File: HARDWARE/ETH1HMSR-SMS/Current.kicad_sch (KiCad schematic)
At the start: 28 parts, among them J501 1710072, U501 HMSR-SMS, U502 DG419LDY, U503 DG411LEDQ, U504 OPA341UA, U505 OPA341UA

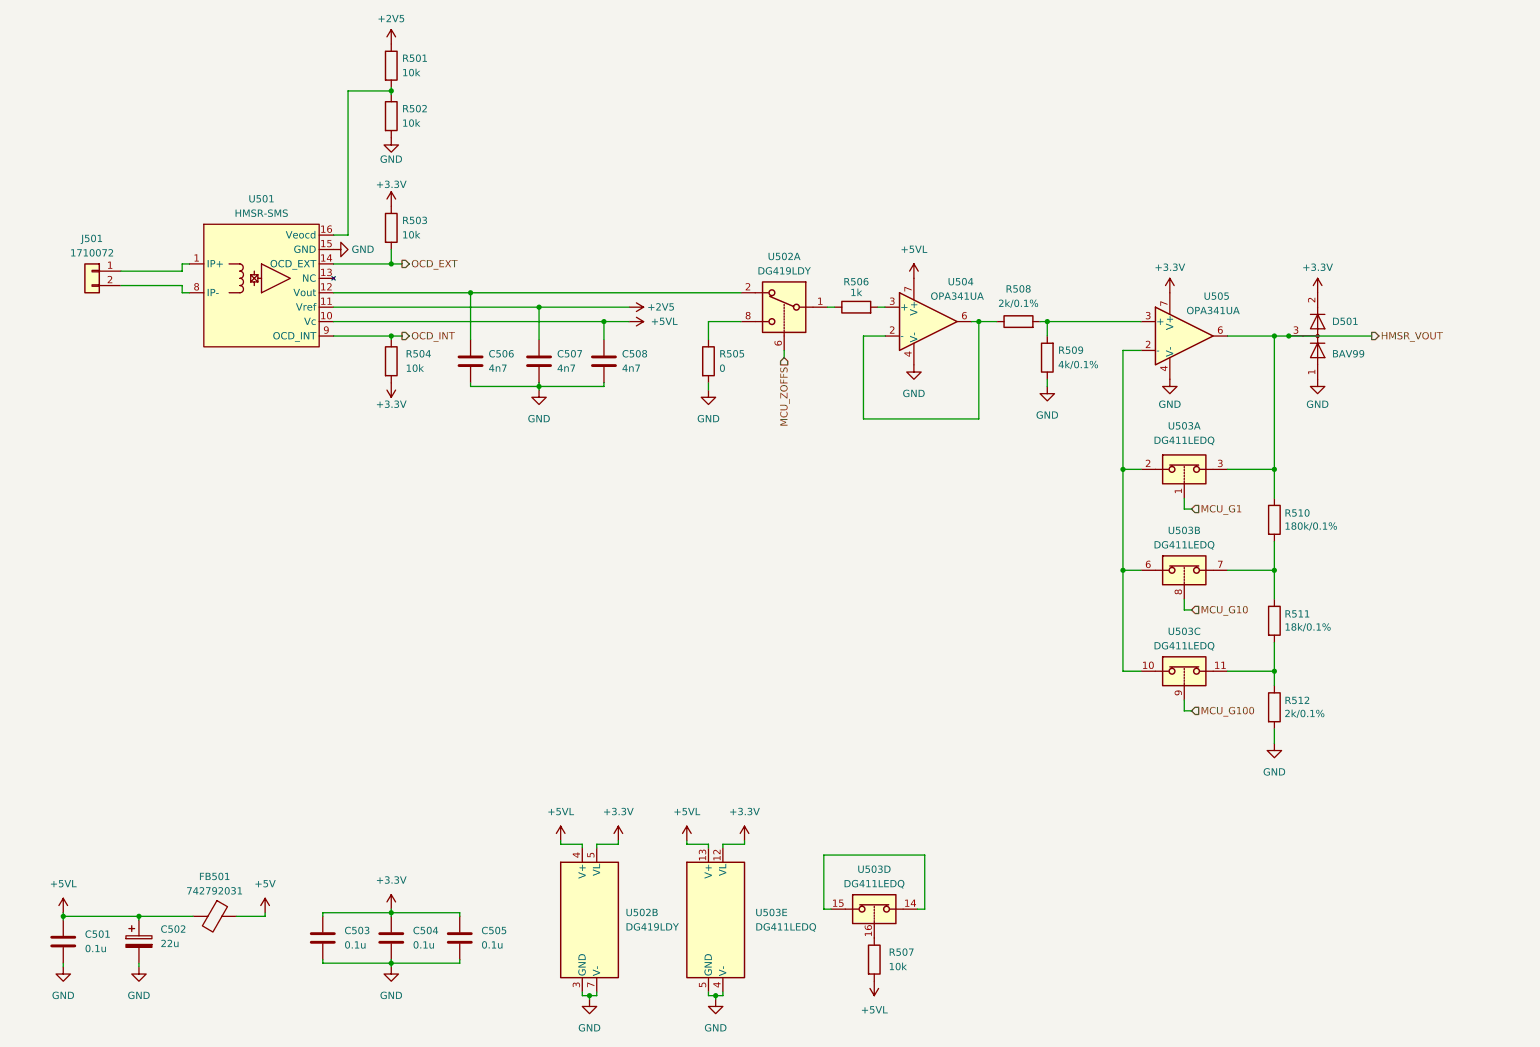
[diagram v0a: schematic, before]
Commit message: SW and HW development
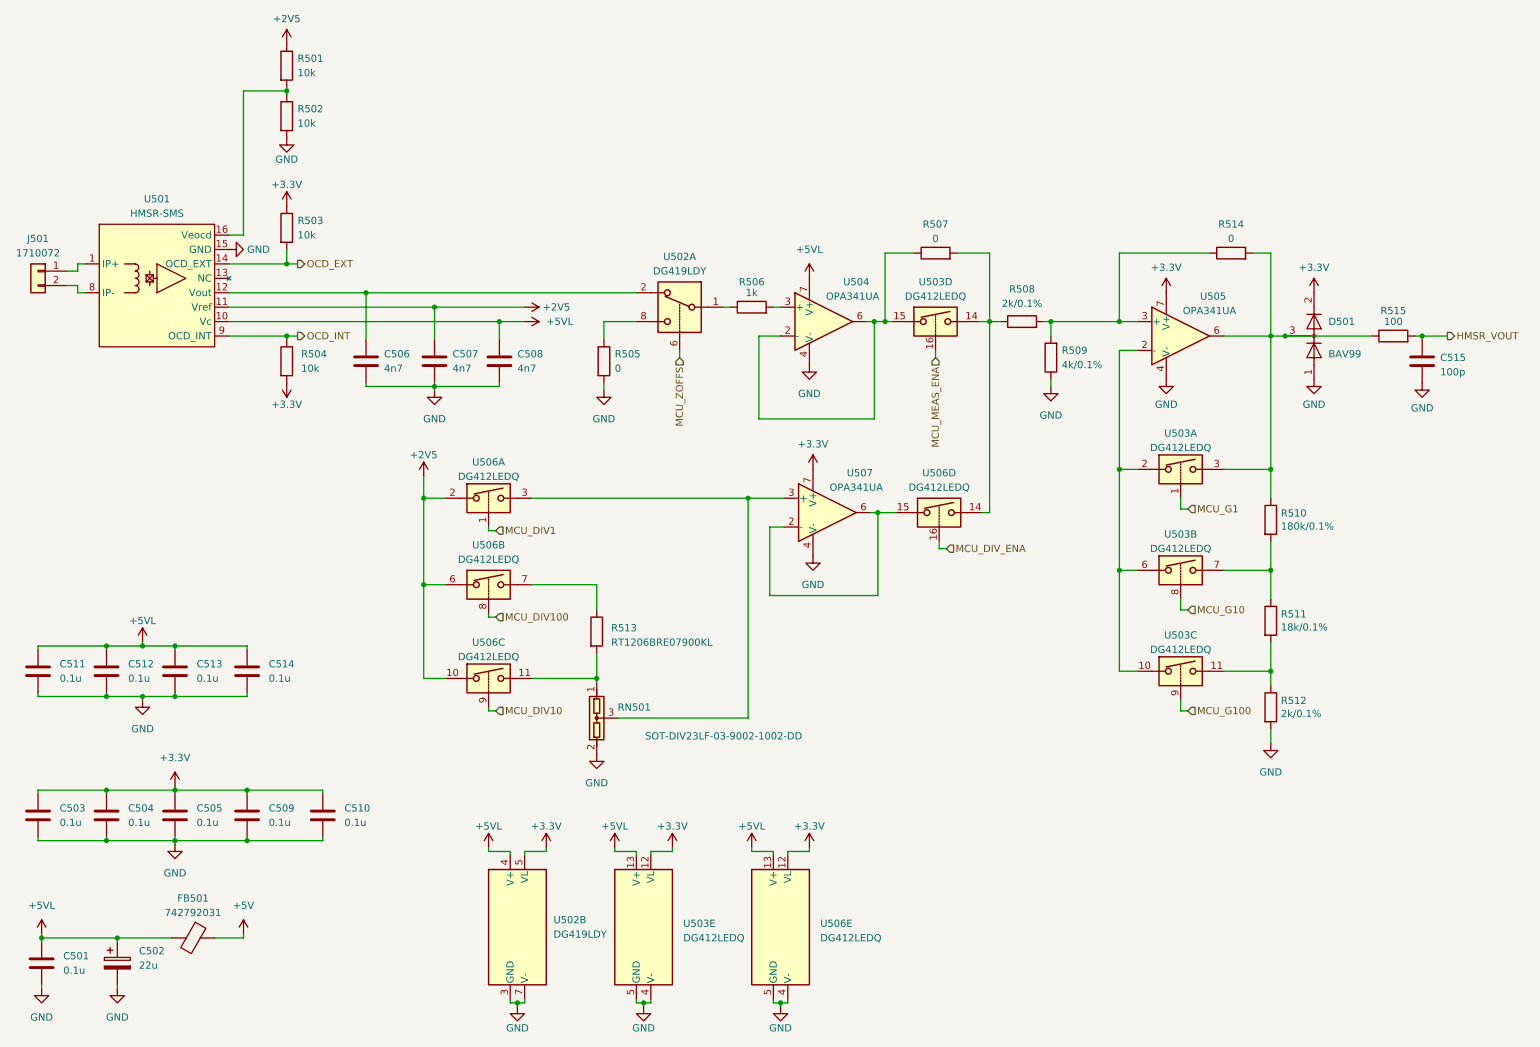
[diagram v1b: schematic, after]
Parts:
- removed U503: DG411LEDQ, Package_SO:TSSOP-16_4.4x5mm_P0.65mm, symbol Analog_Switch:DG411xUE
- added C509, C510, C511, C512, C513, C514: 0.1u, Capacitor_SMD:C_0603_1608Metric_Pad1.08x0.95mm_HandSolder, symbol Device:C
- added C515: 100p, Capacitor_SMD:C_0603_1608Metric_Pad1.08x0.95mm_HandSolder, symbol Device:C
- added R513: RT1206BRE07900KL, Resistor_SMD:R_1206_3216Metric_Pad1.30x1.75mm_HandSolder, symbol Device:R
- added R514: 0, Resistor_SMD:R_0603_1608Metric_Pad0.98x0.95mm_HandSolder, symbol Device:R
- added R515: 100, Resistor_SMD:R_0603_1608Metric_Pad0.98x0.95mm_HandSolder, symbol Device:R
- added RN501: SOT-DIV23LF-03-9002-1002-DD, Package_TO_SOT_SMD:SOT-23, symbol Device:VoltageDivider_CenterPin3
- added U503, U506: DG412LEDQ, Package_SO:TSSOP-16_4.4x5mm_P0.65mm, symbol Analog_Switch:DG412xUE
- added U507: OPA341UA, Package_SO:SOIC-8_3.9x4.9mm_P1.27mm, symbol Amplifier_Operational:OPA340UA
- R507: value 10k -> 0
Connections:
- net +2V5: now also U506.10, U506.2, U506.6
- net +3.3V: now also C509.1, C510.1, U503.12 (VL), U506.12 (VL), U507.7 (V+)
- net +5VL: now also C511.1, C512.1, C513.1, C514.1, U503.13 (V+), U506.13 (V+); no longer R507.2
- net GND: now also C509.2, C510.2, C511.2, C512.2, C513.2, C514.2, C515.2, RN501.2, U503.4 (V-), U503.5 (GND), U506.4 (V-), U506.5 (GND), U507.4 (V-)
- net HMSR_VOUT: now also C515.1, R515.2; no longer D501.3 (K), R510.1, U505.6
- net MCU_G1: now also U503.1
- net MCU_G10: now also U503.8
- net MCU_G100: now also U503.9
- net at R510.2, R511.1: now also U503.7
- net at R511.2, R512.1: now also U503.11
- net at U505.2 (-): now also U503.10, U503.2, U503.6
- net at R508.2, R509.2, U505.3 (+): now also R514.1
- net at R507.1: now also U504.2 (-), U504.6, U503.15
- new net: D501.3 (K), R510.1, R514.2, R515.1, U503.3, U505.6
- new net: U506.15, U507.2 (-), U507.6
- new net: RN501.3, U506.3, U507.3 (+)
- new net: R507.2, R508.1, U503.14, U506.14
- new net: R513.1, U506.7
- new net: R513.2, RN501.1, U506.11
- new net MCU_DIV1: U506.1
- new net MCU_DIV10: U506.9
- new net MCU_DIV100: U506.8
- new net MCU_DIV_ENA: U506.16
- new net MCU_MEAS_ENA: U503.16
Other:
- moved on the sheet: C501, C502, C503, C504, C505, C506, C507, C508, D501, FB501, J501, R501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
